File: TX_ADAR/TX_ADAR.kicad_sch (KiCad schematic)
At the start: 20 parts, among them J19 Conn_Coaxial, J20 Conn_Coaxial, U2 ADAR2001ACCZ

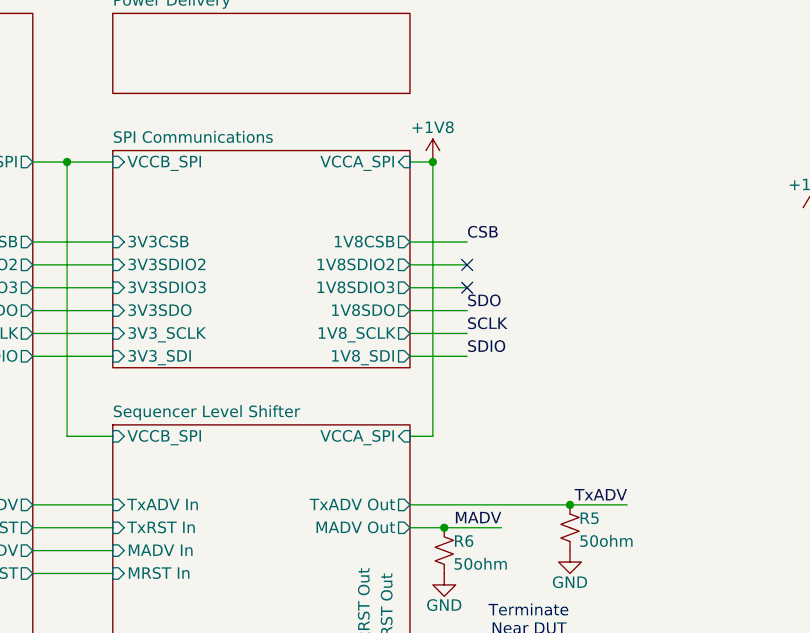
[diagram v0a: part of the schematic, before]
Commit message: Layout Updates
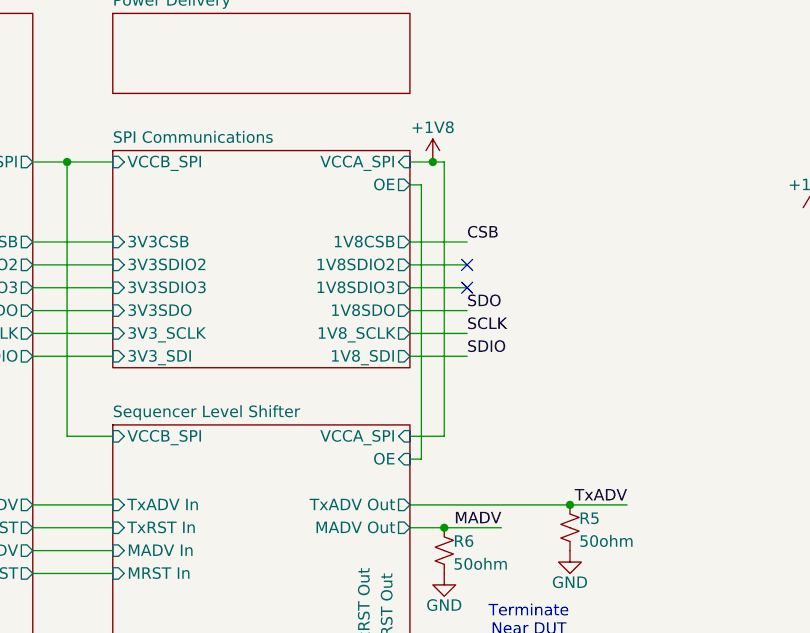
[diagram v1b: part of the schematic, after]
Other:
- sheet SPI Communications ports: added OE; removed none
- sheet Sequencer Level Shifter ports: added OE; removed none
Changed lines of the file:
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@@
 	)
 	(junction
+		(at 90.17 31.75)
+		(diameter 0)
+		(color 0 0 0 0)
+	)
+	(junction
 		(at 231.14 33.02)
 		(diameter 0)
@@
 	)
 	(junction
-		(at 90.17 31.75)
-		(diameter 0)
-		(color 0 0 0 0)
-	)
-	(junction
 		(at 231.14 68.58)
 		(diameter 0)
@@
 	(wire
 		(pts
+			(xy 91.44 31.75) (xy 90.17 31.75)
+		)
+		(stroke
+			(width 0)
+			(type default)
+		)
+	)
+	(wire
+		(pts
 			(xy 227.33 71.12) (xy 231.14 71.12)
 		)
@@
 	(wire
 		(pts
-			(xy 90.17 31.75) (xy 90.17 62.23)
+			(xy 91.44 31.75) (xy 91.44 62.23)
 		)
 		(stroke
@@
 	(wire
 		(pts
-			(xy 90.17 62.23) (xy 87.63 62.23)
+			(xy 91.44 62.23) (xy 87.63 62.23)
 		)
 		(stroke
@@
 	(wire
 		(pts
+			(xy 88.9 34.29) (xy 88.9 64.77)
+		)
+		(stroke
+			(width 0)
+			(type default)
+		)
+	)
+	(wire
+		(pts
 			(xy 45.72 31.75) (xy 49.53 31.75)
 		)
@@
 	(wire
 		(pts
+			(xy 87.63 64.77) (xy 88.9 64.77)
+		)
+		(stroke
+			(width 0)
+			(type default)
+		)
+	)
+	(wire
+		(pts
 			(xy 231.14 33.02) (xy 227.33 33.02)
 		)
@@
 	(wire
 		(pts
+			(xy 87.63 34.29) (xy 88.9 34.29)
+		)
+		(stroke
+			(width 0)
+			(type default)
+		)
+	)
+	(wire
+		(pts
 			(xy 176.53 27.94) (xy 172.72 27.94)
 		)
@@
 			)
 		)
+		(pin "OE" output
+			(at 87.63 34.29 0)
+			(effects
+				(font
+					(size 1.27 1.27)
+				)
+				(justify right)
+			)
+		)
 		(instances
 			(project "TX_ADAR"
@@
 			)
 		)
+		(pin "OE" input
+			(at 87.63 64.77 0)
+			(effects
+				(font
+					(size 1.27 1.27)
+				)
+				(justify right)
+			)
+		)

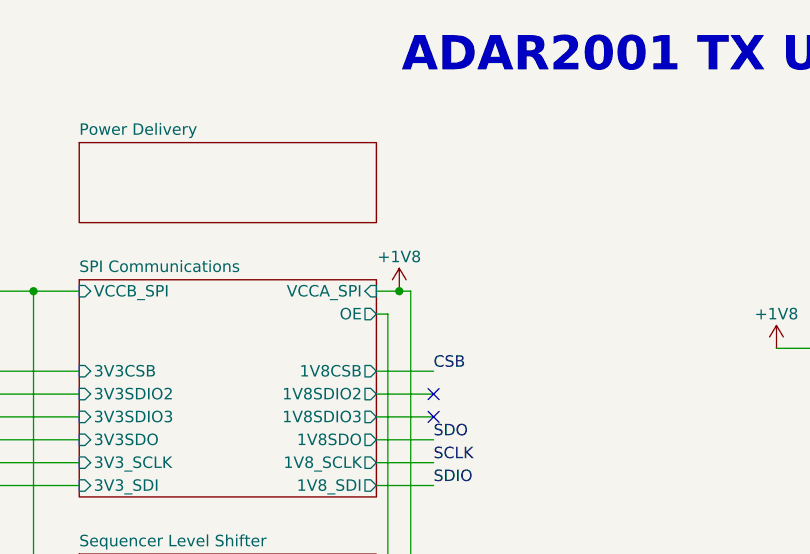
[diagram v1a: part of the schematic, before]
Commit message: Layout comments and slight changes
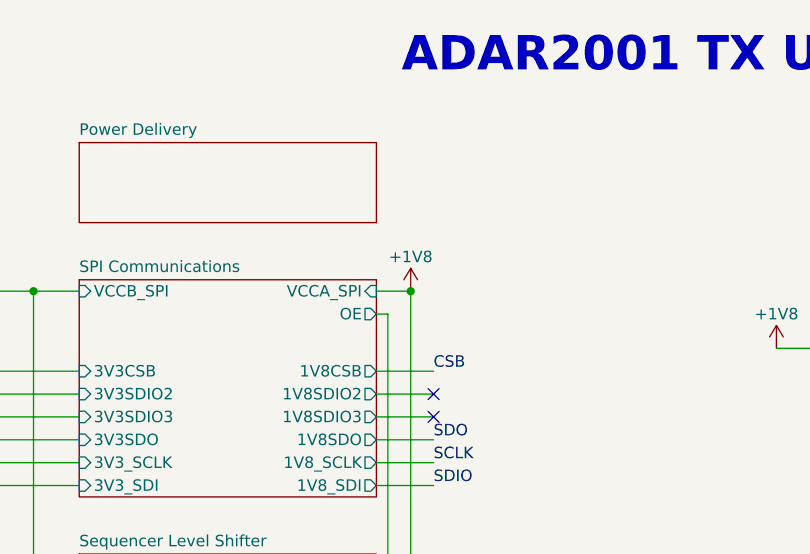
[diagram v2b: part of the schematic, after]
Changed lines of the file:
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@@
 	)
 	(junction
-		(at 90.17 31.75)
+		(at 91.44 31.75)
 		(diameter 0)
 		(color 0 0 0 0)
@@
 	(wire
 		(pts
-			(xy 91.44 31.75) (xy 90.17 31.75)
-		)
-		(stroke
-			(width 0)
-			(type default)
-		)
-	)
-	(wire
-		(pts
 			(xy 227.33 71.12) (xy 231.14 71.12)
 		)
@@
 	(wire
 		(pts
-			(xy 90.17 31.75) (xy 87.63 31.75)
+			(xy 87.63 31.75) (xy 91.44 31.75)
 		)
 		(stroke
@@
 	(symbol
 		(lib_id "power:+1V8")
-		(at 90.17 31.75 0)
+		(at 91.44 31.75 0)
 		(unit 1)
 		(body_style 1)
@@
 		(dnp no)
 		(property "Reference" "#PWR02"
-			(at 90.17 35.56 0)
+			(at 91.44 35.56 0)
 			(hide yes)
 			(show_name no)
@@
 		)
 		(property "Value" "+1V8"
-			(at 90.17 27.94 0)
+			(at 91.44 27.94 0)
 			(show_name no)
 			(do_not_autoplace no)
@@
 		)
 		(property "Footprint" ""
-			(at 90.17 31.75 0)
+			(at 91.44 31.75 0)
 			(hide yes)
 			(show_name no)
@@
 		)
 		(property "Datasheet" ""
-			(at 90.17 31.75 0)
+			(at 91.44 31.75 0)
 			(hide yes)
 			(show_name no)
@@
 		)
 		(property "Description" "Power symbol creates a global label with name \"+1V8\""
-			(at 90.17 31.75 0)
+			(at 91.44 31.75 0)
 			(hide yes)
 			(show_name no)
